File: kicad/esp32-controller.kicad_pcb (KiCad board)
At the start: 2 copper layers, 100 x 70 mm, 55 parts, among them J1 Conn_01x08_Socket, P1 USB_C_Plug_USB2.0, Q1 BCW66G, Q2 BCW66G, Q3 Si2319CDS, SW1 RESET, SW2 BOOT, U1 ESP32-WROVER-IB, U10 Switch, U11 Battery, U12 AP2112K-3.3, U2 Joystick Analog, U3 Joystick Analog, U4 CH340C, U5 TP4056-42-ESOP8, U6 USBLC6-2P6, U7 U8205A, U8 DW01A, U9 LTC4412

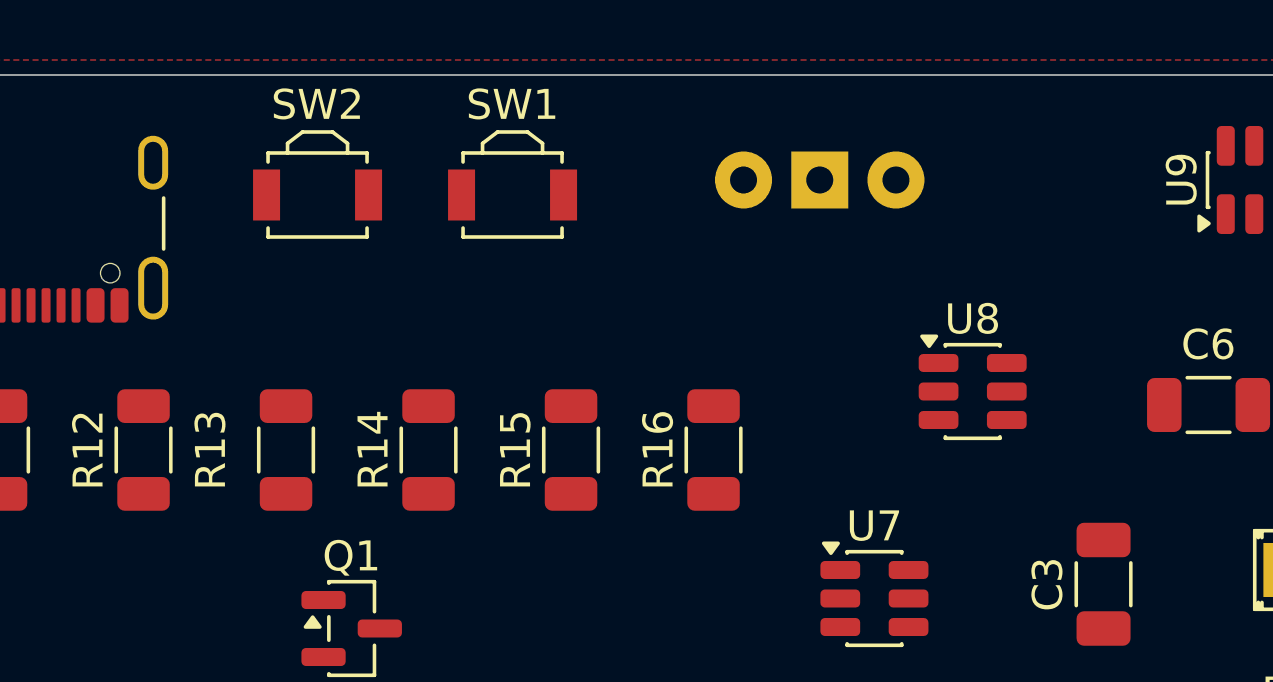
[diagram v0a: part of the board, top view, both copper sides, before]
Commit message: docu
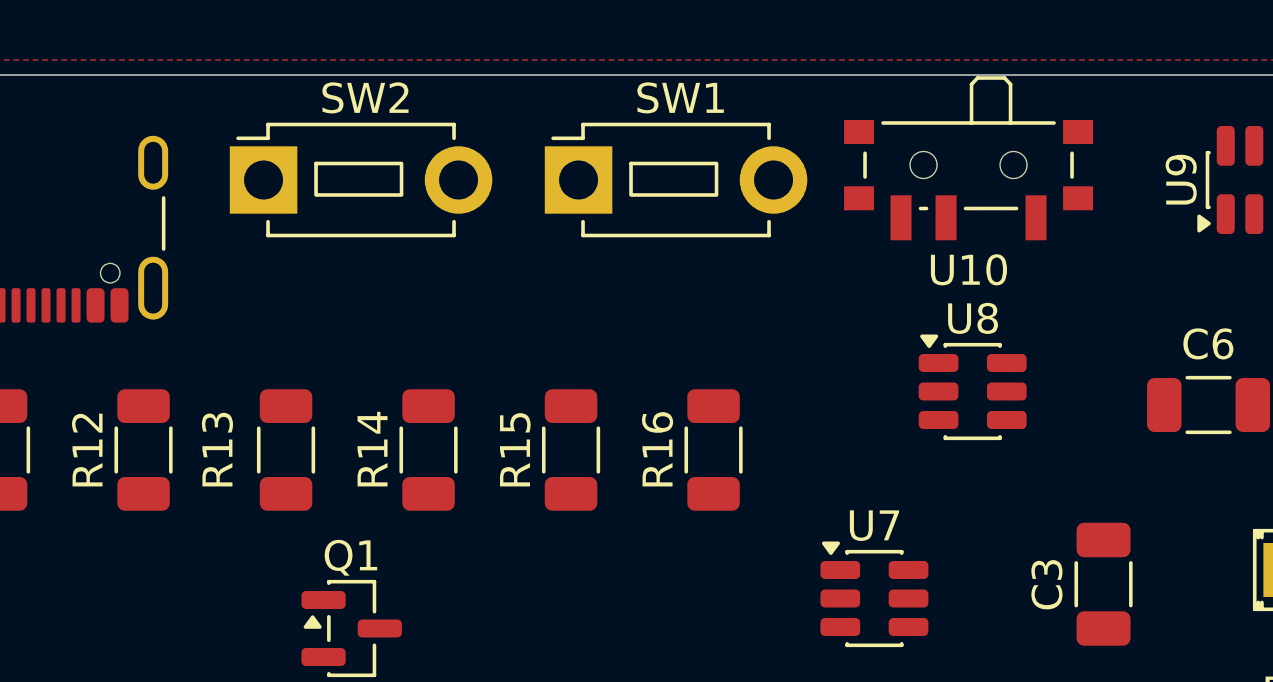
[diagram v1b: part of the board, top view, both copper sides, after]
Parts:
- SW1, SW2: footprint Button_Switch_SMD:SW_SPST_B3U-3000P -> Button_Switch_THT:SW_PUSH_1P1T_6x3.5mm_H4.3_APEM_MJTP1243
- U10: footprint PCM_yvolodym:Switch -> Button_Switch_SMD:SW_SPDT_PCM12; moved to F.Cu
- moved U10 7.50 mm to (175.5, 63.8), turned to 180 degrees
- moved SW1 2.26 mm to (162.5, 64.0)
- moved SW2 1.87 mm to (152.0, 64.0)
